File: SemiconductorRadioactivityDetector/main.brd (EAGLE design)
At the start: 27 parts, among them IC1 4011D, J1 22-05-7028-02, J2 22-05-7028-02, J3 22-05-7028-02, Q1 IRF530

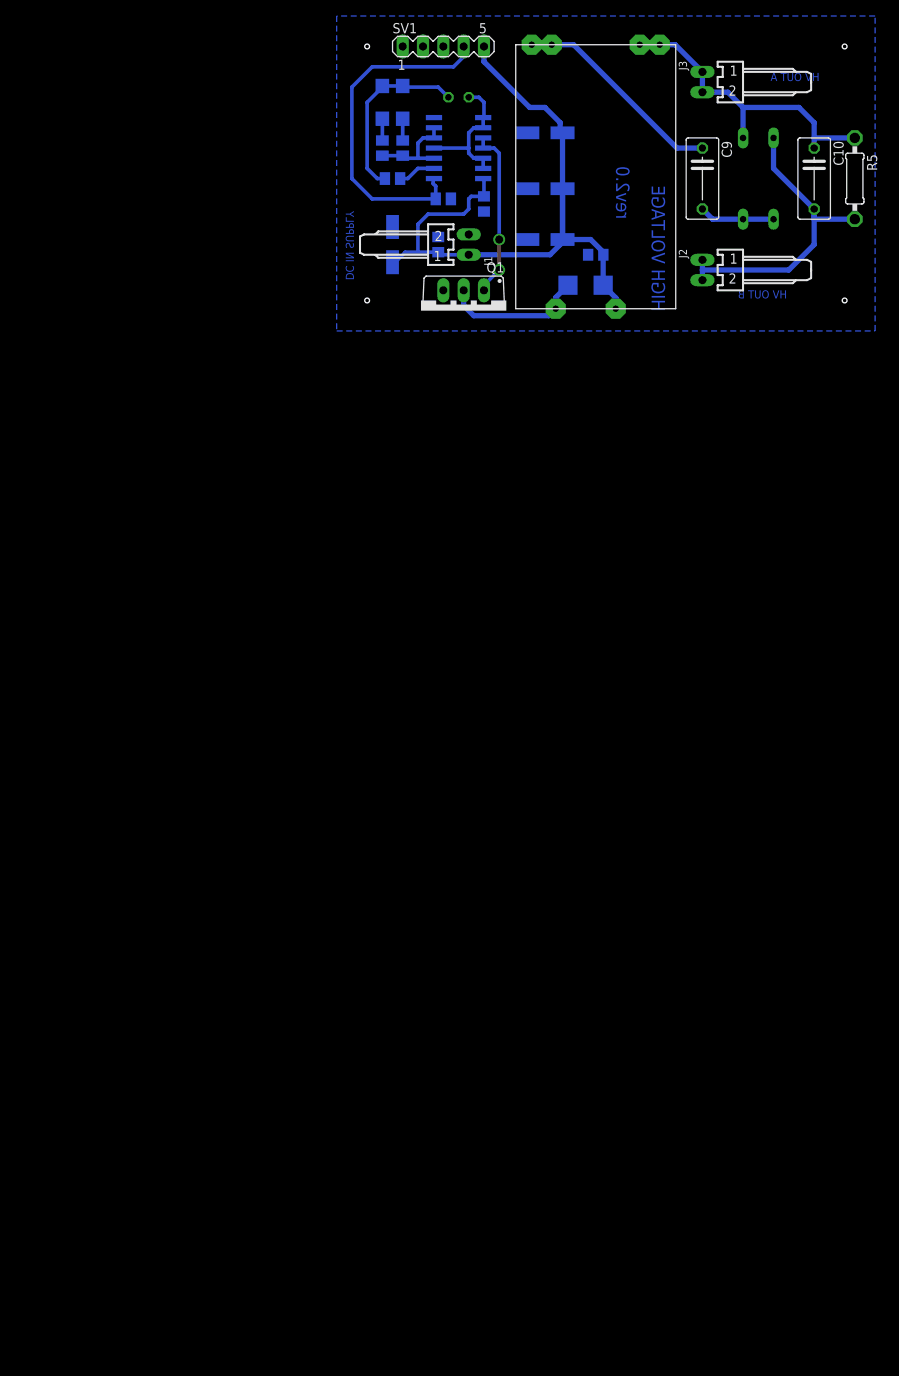
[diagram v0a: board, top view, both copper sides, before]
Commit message: Initial unfinished version.
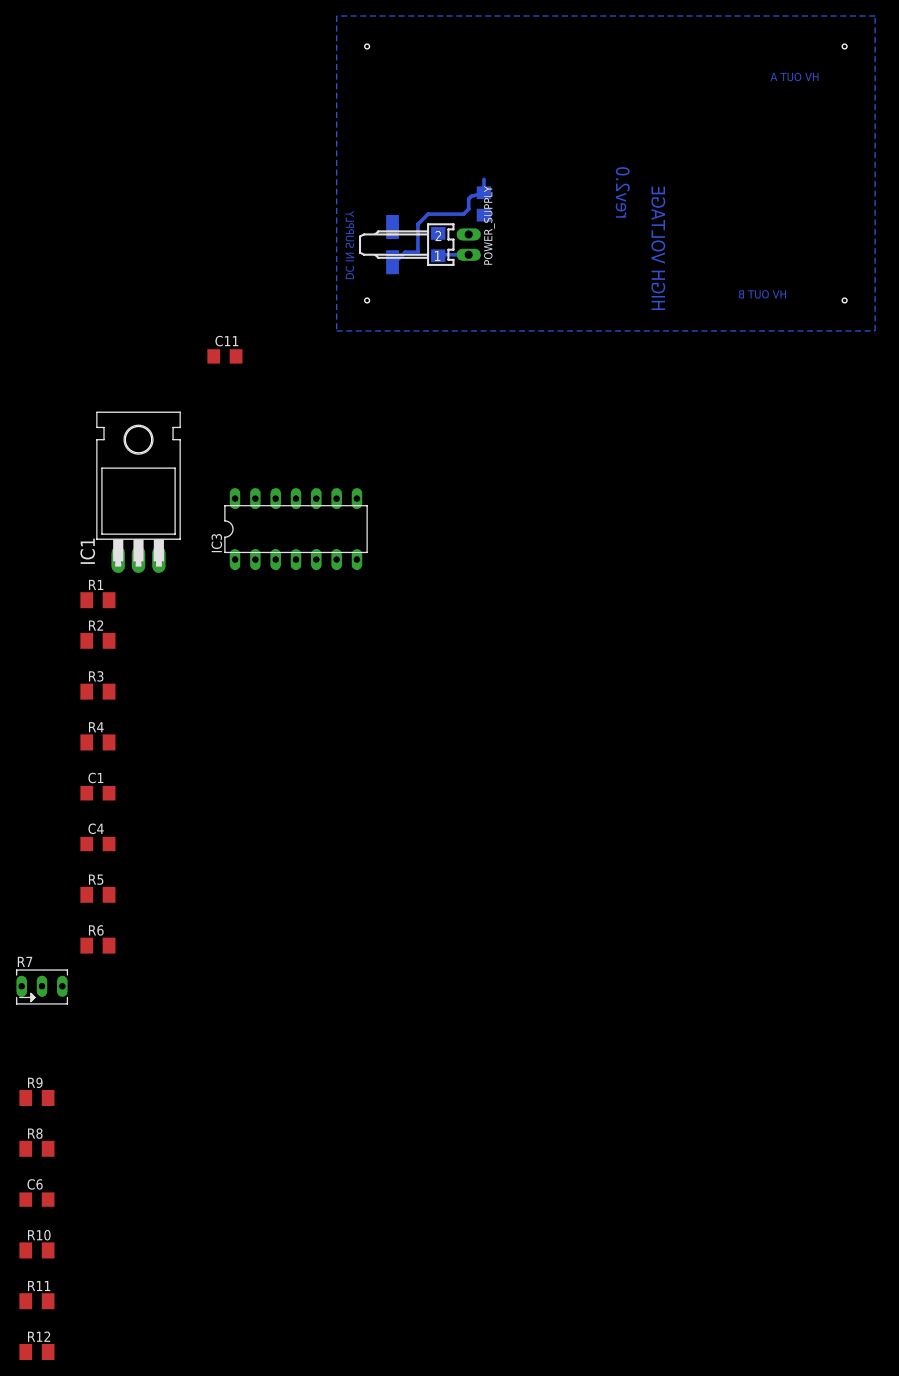
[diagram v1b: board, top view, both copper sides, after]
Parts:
- removed 11: CCFL_INVERTER_COIL, ccfl_inverter_coil:CCFL_INVERTER_COIL
- removed C10: 2n2/4k, resistor:C075-042X103
- removed C5: 100u/16V, resistor:153CLV-0505
- removed C8: 220n, resistor:C0805
- removed C9: 2n2/4k, rcl:C075-042X103
- removed D1, D2: GF1, diode:SMA-DO214AC
- removed D3: ES2D, diode:SMB
- removed D4, D5: BAV21, diode:DO35-10
- removed J2, J3: 22-05-7028-02, con-molex:7395-02
- removed Q1: IRF530, transistor-power:TO220BV
- removed SV1: (no value), con-lstb:MA05-1
- added C11: 100n, resistor:C1206
- added IC3: LM324N, linear:DIL14
- added R10, R11, R12, R6, R8, R9: 2k, resistor:M1206
- added R7: (no value), pot:B64Y
- C1: value 220n -> 100n; device resistor:C025-025X050 -> resistor:C1206
- C2: device resistor:C0805 -> resistor:C1206
- C4, C6: value 100u/16V -> 100n; device rcl:153CLV-0505 -> resistor:C1206
- C7: value 220n -> 100n; device resistor:C0805 -> resistor:C1206
- IC1: value 4011D -> 317T; device 40xx:SO14 -> linear:TO220H
- R1: value 4k7 -> 240R; device resistor:M0805 -> resistor:M1206
- R2, R3, R4: value 2k2 -> 2k; device resistor:M0805 -> resistor:M1206
- R5: value 33M -> 2k; device resistor:0207/10 -> resistor:M1206
- moved C6 147.7 mm to (-37.5, -108.6), flipped to the top, turned to 0 degrees
- moved R5 130.3 mm to (-29.8, -70.5), turned to 0 degrees
- moved C1 98.0 mm to (-29.8, -57.8), flipped to the top
- moved C4 94.0 mm to (-29.8, -64.1), flipped to the top, turned to 0 degrees
- moved R4 83.5 mm to (-29.8, -51.4), flipped to the top, turned to 0 degrees
- moved R3 76.7 mm to (-29.8, -45.1), flipped to the top, turned to 0 degrees
- moved R2 68.5 mm to (-29.8, -38.7), flipped to the top
- moved R1 66.2 mm to (-29.8, -33.7), flipped to the top
- moved IC1 57.5 mm to (-24.8, -18.4), flipped to the top, turned to 0 degrees
- renumbered J1 to POWER_SUPPLY
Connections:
- removed net N$22: IC1.3, IC1.5, IC1.6, R3.1, R4.1
- removed net N$23: C1.2, D1.A, D2.K, R2.2
- removed net N$24: D1.K, R3.2
- removed net N$25: D2.A, R4.2
- new net N$12: C6.1, IC3.13, R10.2, R11.1
- new net N$13: C6.2, IC3.14, R10.1
- new net N$14: IC3.12, R12.2
- new net N$8: C2.1, C3.+, IC1.3, POWER_SUPPLY.1
- new net N$9: R7.E, R9.2
- net GND: now also C1.2, C11.2, C4.2, IC3.11, R12.1, R2.1, R8.2; no longer C4.-, C5.-, C6.-, C8.2, IC1.7, Q1.S, SV1.1, SV1.2, SV1.3
- net N$1: now also IC1.1, R1.1, R2.2; no longer IC1.2, R2.1
- net N$10: now also R7.A, R8.1; no longer C10.2, D5.C, J2.1, J2.2, R5.2
- net N$11: now also IC3.9, R7.S; no longer 11.S2.A, 11.S2.B, C10.1, D4.A, J3.1, J3.2, R5.1
- net N$2: now also IC3.2, R3.2, R4.2; no longer IC1.1, R1.2, SV1.4
- net N$3: now also IC3.1, IC3.5, R3.1; no longer 11.P2, D3.A, Q1.D
- net N$4: now also C1.1, R4.1; no longer IC1.10, IC1.11, Q1.G
- net N$5: now also IC3.6, R5.2, R6.2; no longer C1.1, IC1.12, IC1.13, IC1.4, IC1.8, IC1.9
- net N$6: now also IC3.10, IC3.7, R11.2, R5.1; no longer 11.S1.A, 11.S1.B, C9.1
- net N$7: now also C4.1, R6.1; no longer C9.2, D4.C, D5.A
- net VCC: now also C11.1, IC1.2, IC3.4, R1.2, R9.1; no longer 11.P1, C2.1, C3.+, C4.+, C5.+, C6.+, C8.1, D3.C, IC1.14, POWER_SUPPLY.1, R1.1, SV1.5
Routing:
- net VCC: track 88.8 -> 19.5 mm
- net N$2: track 42.5 -> 0.00 mm
- net N$10: track 39.6 -> 0.00 mm
- net N$11: track 39.4 -> 0.00 mm
- net N$6: track 26.7 -> 0.00 mm
- net N$23: track 22.7 -> 0.00 mm
- net N$4: track 21.5 -> 0.00 mm, vias 2 -> 0
- net N$3: track 18.2 -> 0.00 mm
- net N$5: track 17.7 -> 0.00 mm
- net N$22: track 12.0 -> 0.00 mm
- net N$7: track 9.42 -> 0.00 mm
- net N$1: track 4.76 -> 0.00 mm
- net N$8: track 0.00 -> 4.25 mm
- net N$25: track 2.71 -> 0.00 mm
- net N$24: track 2.71 -> 0.00 mm
